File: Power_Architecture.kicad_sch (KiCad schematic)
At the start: 0 parts

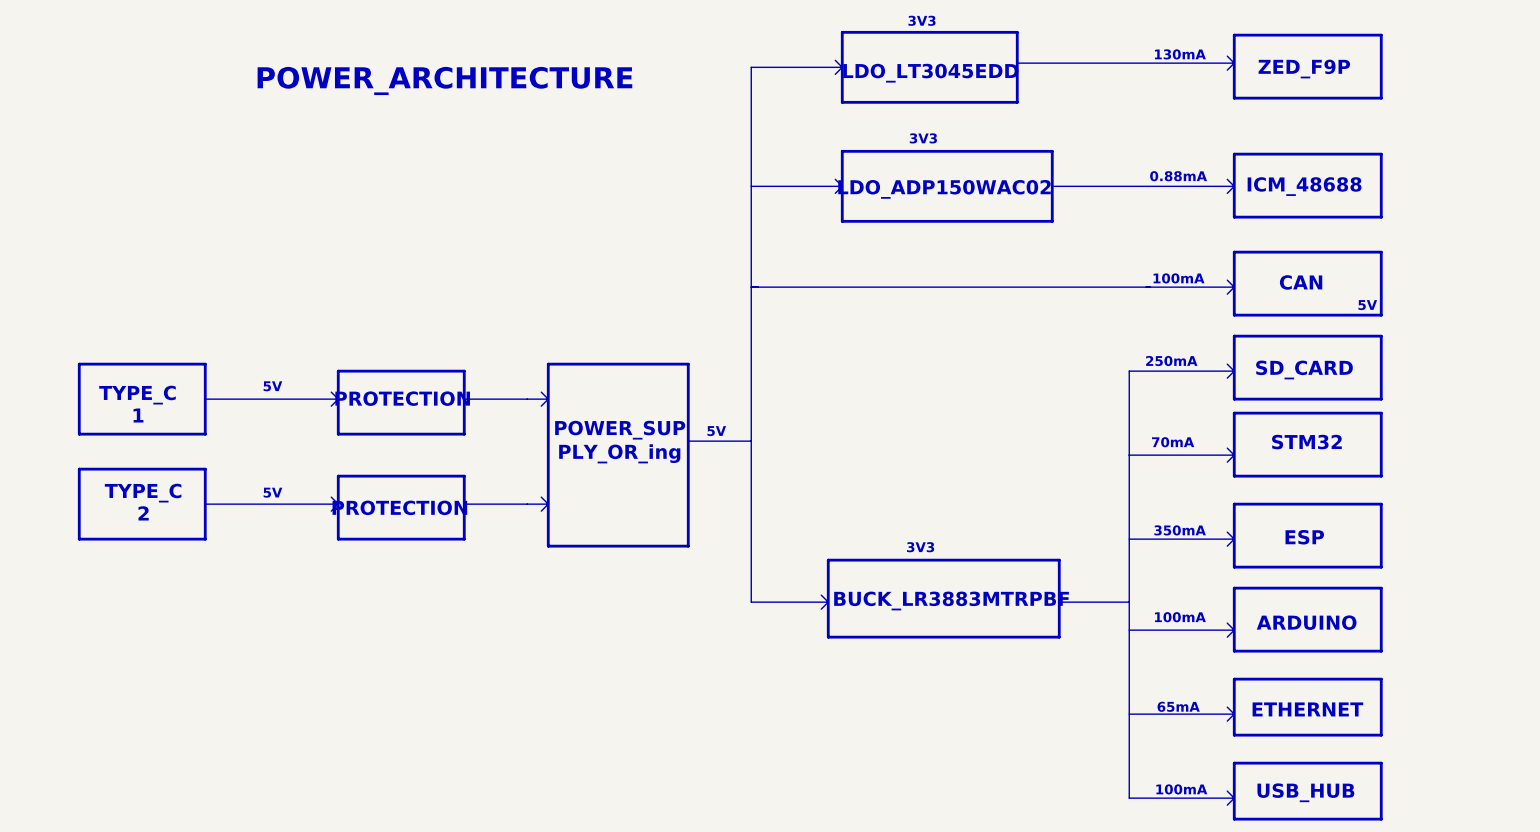
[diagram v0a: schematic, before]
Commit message: we
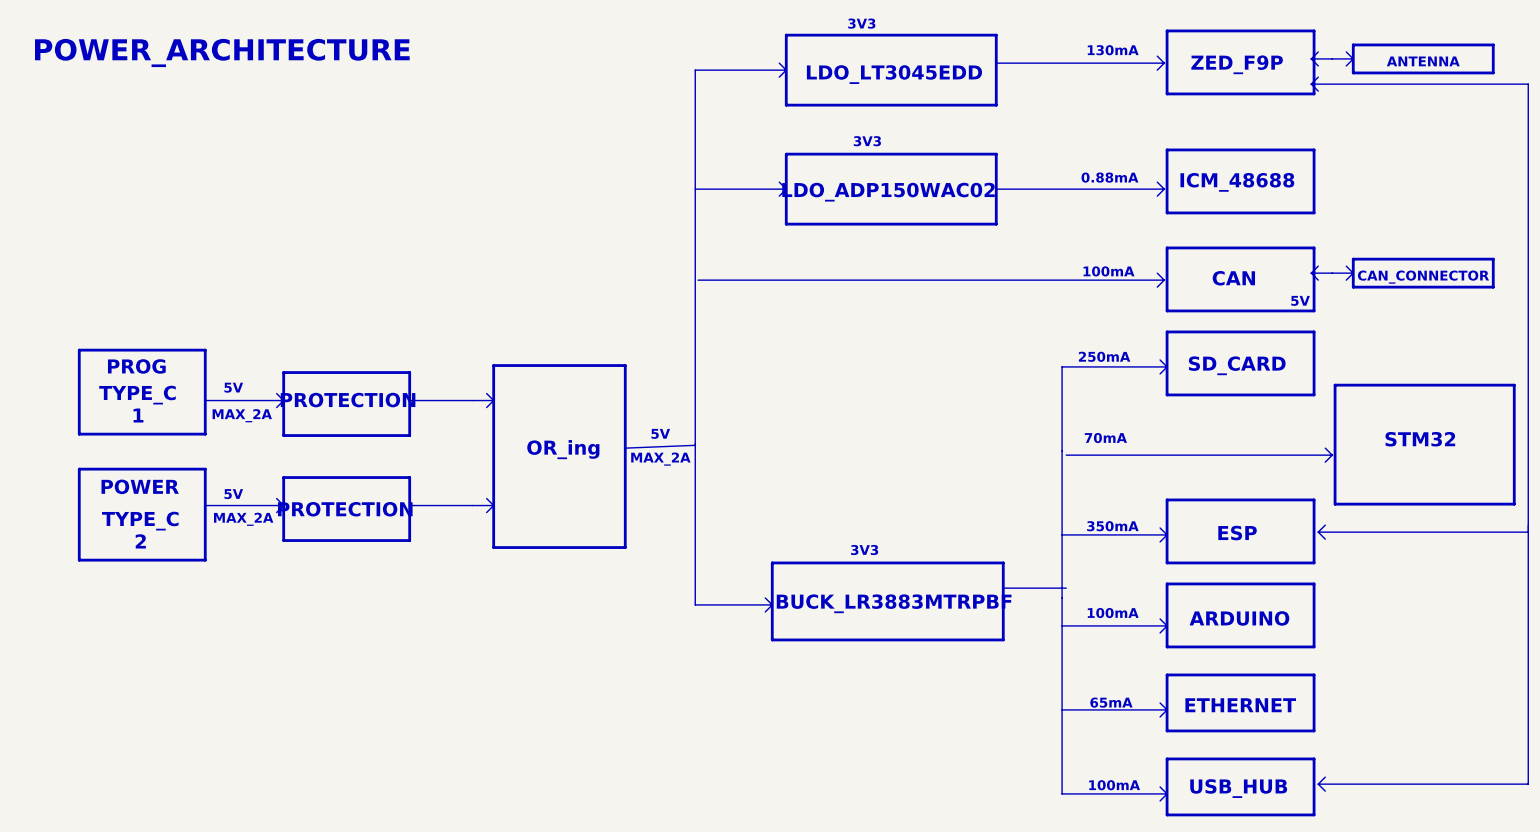
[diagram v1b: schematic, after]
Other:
- note added: "ANTENNA"
- note added: "CAN_CONNECTOR"
- note added: "MAX_2A"
- note added: "OR_ing"
- note added: "POWER"
- note added: "PROG"
- note removed: "PLY_OR_ing"
- note removed: "POWER_SUP"
